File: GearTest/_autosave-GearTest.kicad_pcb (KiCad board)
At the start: 2 copper layers, 62.4 x 113 mm, 21 parts, among them J2 Терминал выключателя моторов, J3 Терминал выключателя основног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, J5 Терминал питания XY-FZ35, J6 Терминал LCD_1602_I2C, J7 Терминал UART1, M1 Motor_DC, M2 Motor_DC, Q1 IRLZ44N, SW1 Выключатель моторов, SW3 SW_Push, U1 WeAct BlackPill STM32F411C_C-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, U2 CH340N, U3 INA219

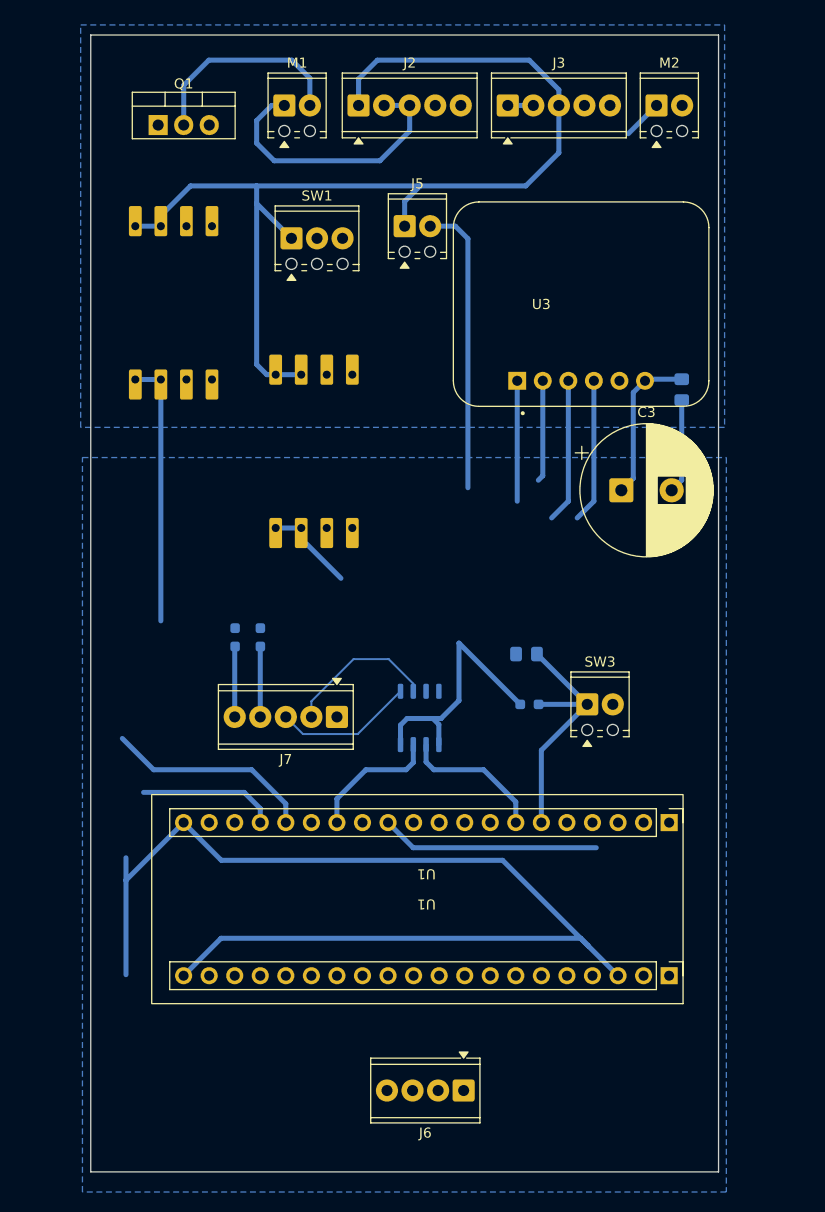
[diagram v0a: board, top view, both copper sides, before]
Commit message: dev
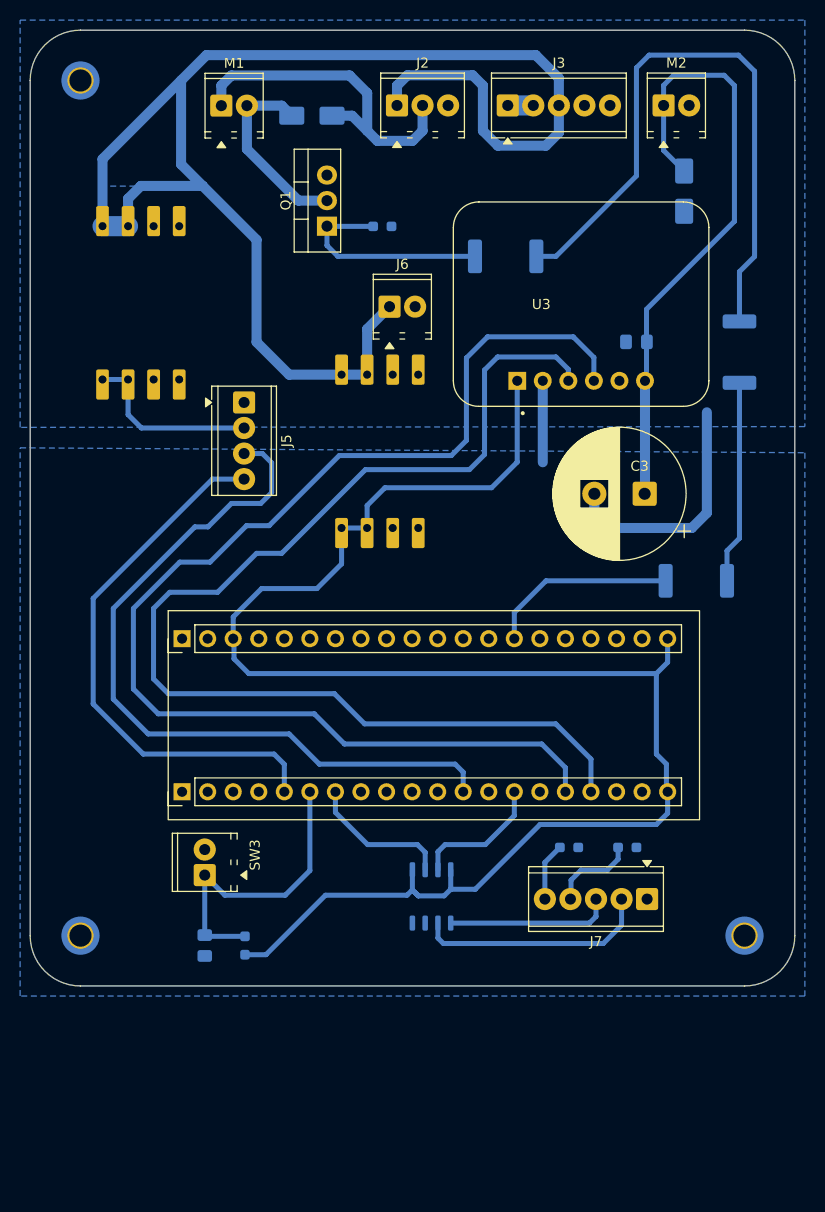
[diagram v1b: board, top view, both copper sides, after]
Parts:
- removed SW1: Выключатель моторов, TerminalBlock_Phoenix:TerminalBlock_Phoenix_MPT-0,5-3-2.54_1x03_P2.54mm_Horizontal
- added D1: SS34, Diode_SMD:D_SMA, B.Cu at (97.7, 53.7)
- added D2: SS34, Diode_SMD:D_SMA, B.Cu at (134.7, 61.2)
- added H1: MountingHole, MountingHole:MountingHole_2.2mm_M2_DIN965_Pad_TopOnly, B.Cu at (74.7, 135.2)
- added H2: MountingHole, MountingHole:MountingHole_2.2mm_M2_DIN965_Pad_TopOnly, B.Cu at (140.7, 135.2)
- added H3: MountingHole, MountingHole:MountingHole_2.2mm_M2_DIN965_Pad_TopOnly, B.Cu at (74.7, 50.2)
- added R1: 0R, Resistor_SMD:R_2512_6332Metric_Pad1.40x3.35mm_HandSolder, B.Cu at (135.9, 99.9)
- added R2: 0R, Resistor_SMD:R_2512_6332Metric_Pad1.40x3.35mm_HandSolder, B.Cu at (140.2, 77.2)
- added R3: 0R, Resistor_SMD:R_2512_6332Metric_Pad1.40x3.35mm_HandSolder, B.Cu at (117.0, 67.6)
- added R4: 10k, Resistor_SMD:R_0603_1608Metric_Pad0.98x0.95mm_HandSolder, B.Cu at (104.7, 64.7)
- J2: footprint TerminalBlock_Phoenix:TerminalBlock_Phoenix_MPT-0,5-5-2.54_1x05_P2.54mm_Horizontal -> TerminalBlock_Phoenix:TerminalBlock_Phoenix_MPT-0,5-3-2.54_1x03_P2.54mm_Horizontal
- moved J5 71.8 mm to (91.0, 82.2), turned to -90 degrees
- moved C1 43.2 mm to (87.1, 136.1), turned to -90 degrees
- moved R6 42.0 mm to (129.1, 126.4), turned to 0 degrees
- moved SW3 41.6 mm to (87.1, 129.1), turned to 90 degrees
- moved R7 39.2 mm to (123.3, 126.4), turned to 0 degrees
- moved R5 37.1 mm to (91.1, 136.1), turned to -90 degrees
- moved J7 35.8 mm to (131.0, 131.5)
- moved Q1 19.6 mm to (99.2, 64.6), turned to 90 degrees
- moved U1 18.3 mm to (108.9, 113.2), turned to 0 degrees
- moved U2 17.8 mm to (109.6, 131.3), turned to 90 degrees
- moved J6 8.14 mm to (105.4, 72.6)
- moved D4 6.55 mm to (104.5, 87.0)
- moved C2 6.54 mm to (130.0, 76.1), turned to 180 degrees
- moved M1 6.26 mm to (88.7, 52.7)
- moved J2 3.82 mm to (106.2, 52.6)
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- renumbered D1 to D3, D2 to D4, J6 to J5, J5 to J6, R2 to R5, R3 to R6, R4 to R7
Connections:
- net Net-(U3-PadVIN-) renamed /L+
- J2 pad 2: Net-(J2-Pin_2) -> Net-(D1-A)
- J2 pad 3: Net-(J2-Pin_2) -> GNDPWR
- J5 pad 1: GNDD -> GNDPWR
- J6 pad 2: GNDD -> GNDPWR
- M1 pad 1: Net-(J2-Pin_2) -> Net-(D1-A)
- Q1 pad 1: /MOTOR_GATE -> Net-(Q1-G)
- U1 pad 11: unconnected-(U1-PA1-Pad11) -> /MOTOR_GATE
- U1 pad 33: /MOTOR_GATE -> unconnected-(U1-PA12-Pad33)
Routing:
- net /INA219_MOTOR_SDA: track 28.0 -> 115.2 mm
- net /INA219_MOTOR_SCL: track 35.1 -> 121.5 mm
- net Net-(R2-Pad2): track 0.00 -> 62.4 mm
- net /LCD1602_MOTOR_SCL: track 0.00 -> 54.6 mm
- net /LCD1602_MOTOR_SDA: track 21.7 -> 75.3 mm
- net 12V0: track 107.6 -> 149.6 mm
- net Net-(D2-K): track 19.5 -> 61.3 mm
- net Net-(D1-A): track 0.00 -> 34.4 mm
- net GNDD: track 39.1 -> 8.10 mm
- net Net-(J2-Pin_2): track 27.9 -> 0.00 mm
- net Net-(Q1-G): track 0.00 -> 21.6 mm
- net Net-(R1-Pad2): track 0.00 -> 20.2 mm
- net /MOTOR_GATE: track 0.00 -> 18.9 mm
- net GNDPWR: track 9.38 -> 24.4 mm
- net 5V0: track 26.5 -> 16.6 mm
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- added copper zone on B.Cu, net 12V0
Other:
- board size 62.4 x 113 mm -> 76 x 95 mm
